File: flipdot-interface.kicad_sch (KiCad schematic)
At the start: 58 parts, among them J1 Conn_02x30_Odd_Even, J2 Conn_02x06_Odd_Even, J3 Screw_Terminal_01x04, J4 Conn_02x06_Odd_Even, U10 74LVC1G19, U11 74HCT595, U12 ULN2803A, U13 74HCT244, U14 LM2734Y

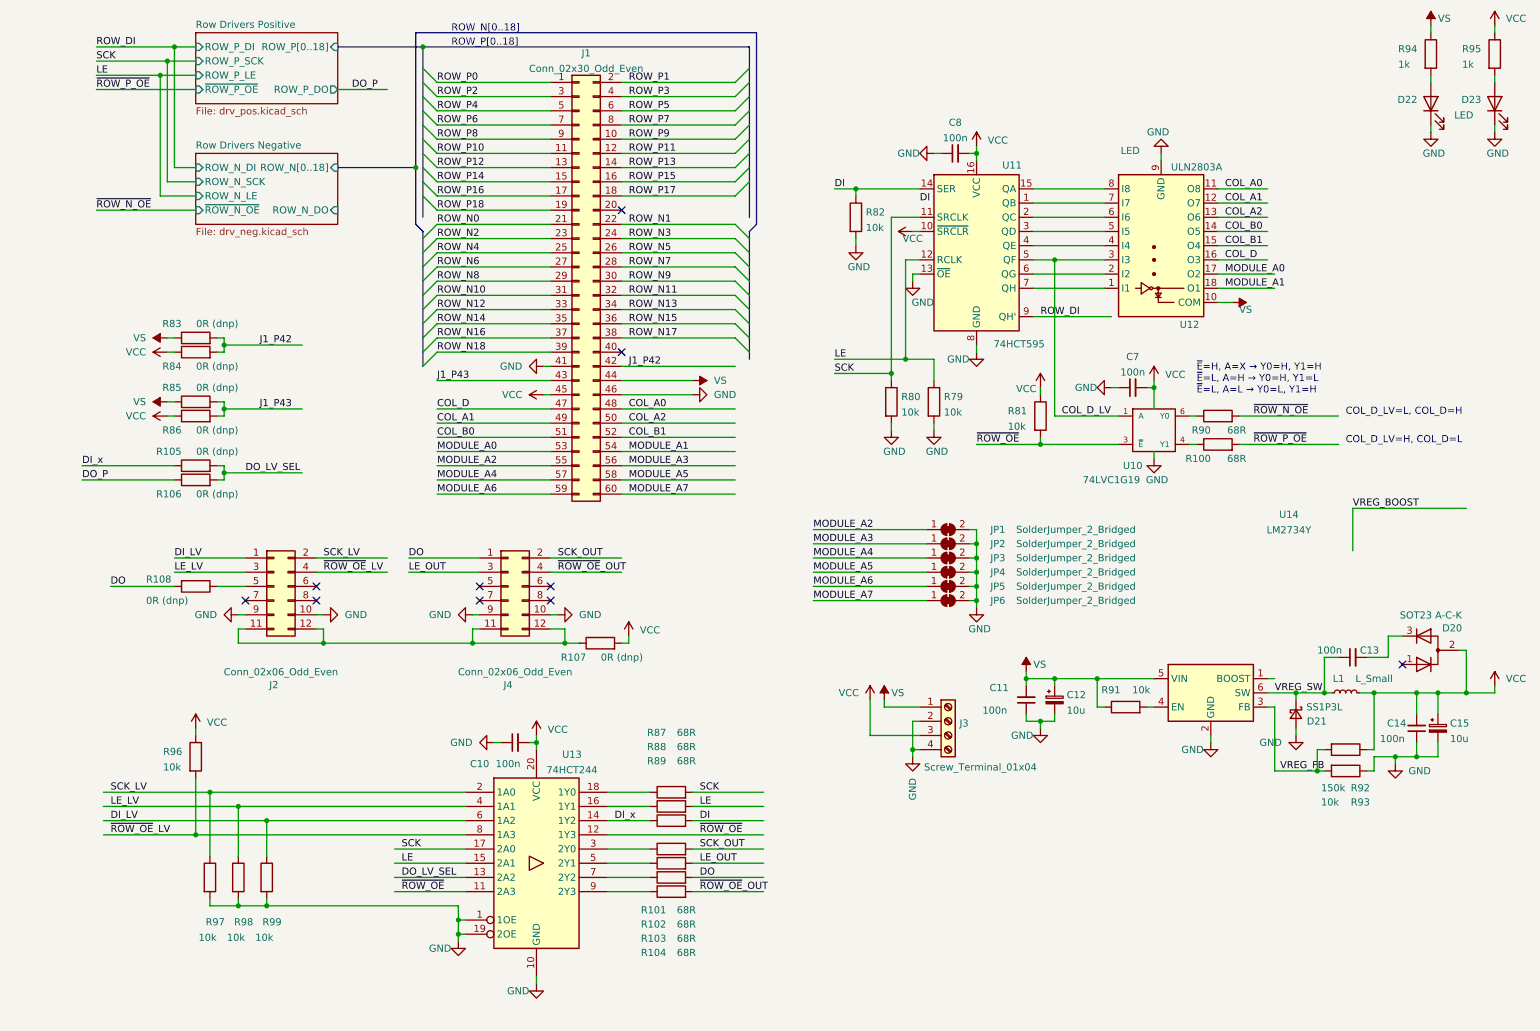
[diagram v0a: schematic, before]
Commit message: More work, moved digital stuff to sub-schematic.
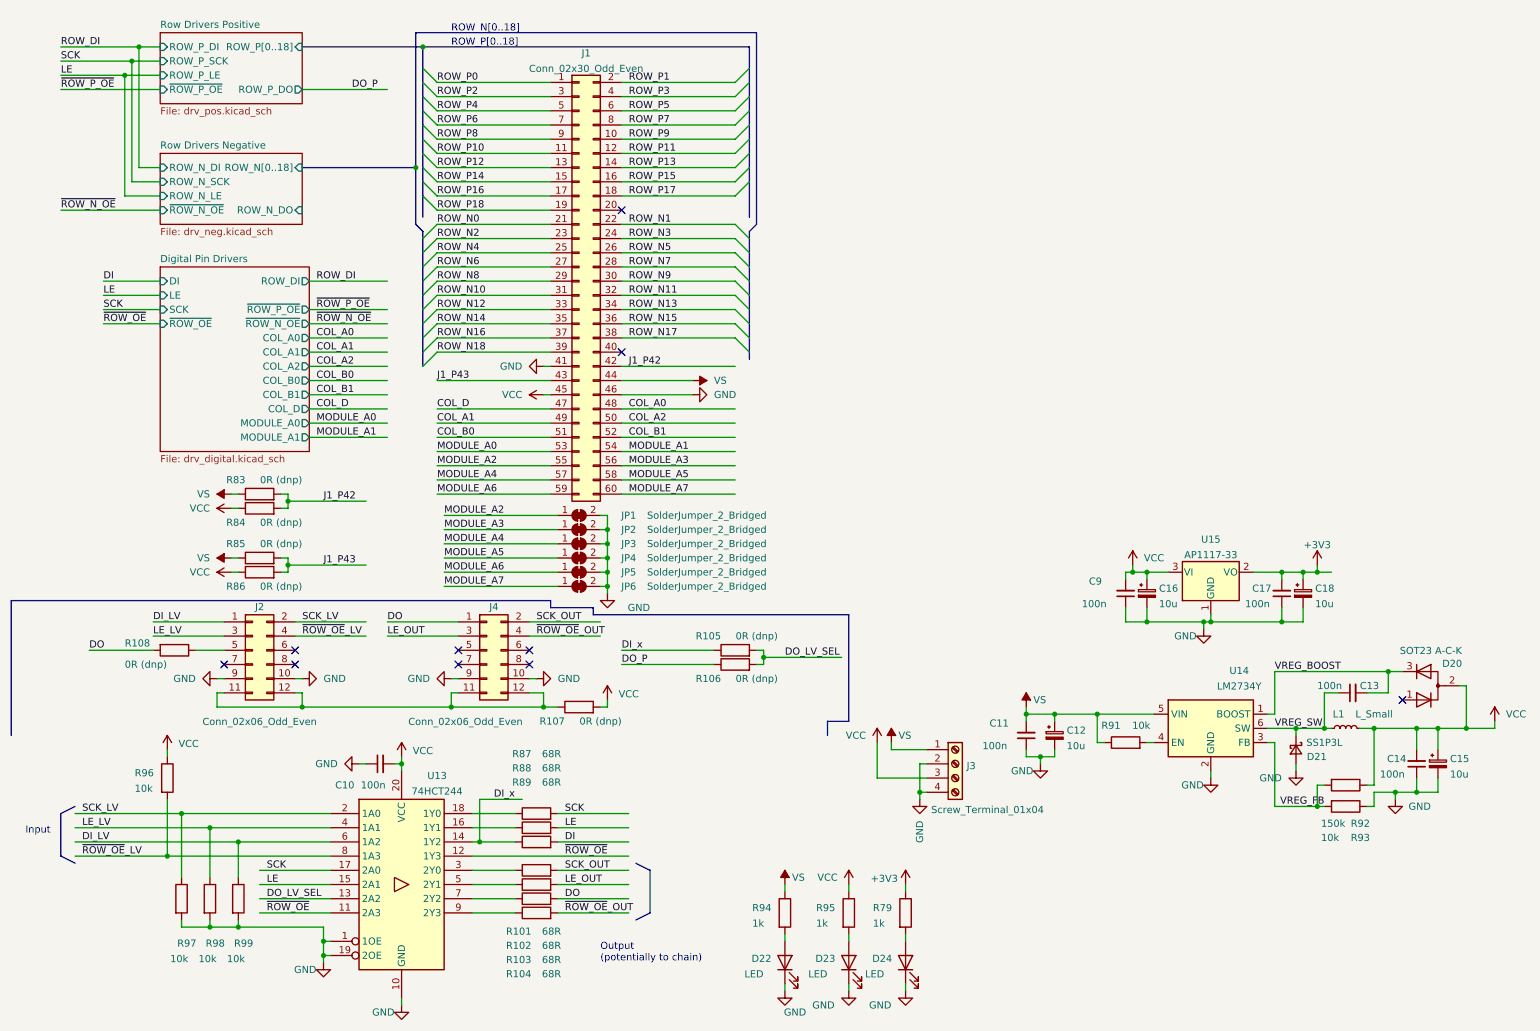
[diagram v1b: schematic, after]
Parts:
- removed C7, C8: 100n, Capacitor_SMD:C_0603_1608Metric, symbol Device:C_Small
- removed R100, R90: 68R, Resistor_SMD:R_0603_1608Metric, symbol Device:R
- removed R80, R81, R82: 10k, Resistor_SMD:R_0603_1608Metric, symbol Device:R
- removed U10: 74LVC1G19, Package_TO_SOT_SMD:SOT-563, symbol 74xGxx:74LVC1G19
- removed U11: 74HCT595, Package_SO:SOIC-16_3.9x9.9mm_P1.27mm, symbol 74xx:74HCT595
- removed U12: ULN2803A, Package_SO:SOIC-18W_7.5x11.6mm_P1.27mm, symbol Transistor_Array:ULN2803A
- added C16, C18: 10u, Capacitor_Tantalum_SMD:CP_EIA-3216-18_Kemet-A, symbol Device:C_Polarized_Small
- added C17, C9: 100n, Capacitor_SMD:C_0603_1608Metric, symbol Device:C_Small
- added D24: LED, LED_SMD:LED_0603_1608Metric, symbol Device:LED
- added U15: AP1117-33, Package_TO_SOT_SMD:SOT-223-3_TabPin2, symbol Regulator_Linear:AP1117-33
- R79: value 10k -> 1k
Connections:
- net GND: now also C16.2, C17.1, C18.2, C9.1, D24.1 (K), U15.1 (GND); no longer R79.2
- net LE: no longer R79.1
- net VCC: now also C16.1, C9.2, U15.3 (VI)
- net VREG_BOOST: now also C13.2, D20.3 (K), U14.1 (BOOST)
- new net: D24.2 (A), R79.2
- new net +3V3: C17.2, C18.1, R79.1, U15.2 (VO)
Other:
- added sheet Digital Pin Drivers (drv_digital.kicad_sch)
- note added: "Input"
- note added: "Output (potentially to chain)"
- note removed: "COL_D_LV=H, COL_D=L"
- note removed: "COL_D_LV=L, COL_D=H"
- note removed: "~{E}=H, A=X → Y0=H, Y1=H ~{E}=L, A=H → Y0=H, Y1=L ~{E}=L, A=L → Y0=L, Y1=H"
- moved on the sheet: C10, C11, C12, C13, C14, C15, D20, D21, D22, D23, J2, J3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
